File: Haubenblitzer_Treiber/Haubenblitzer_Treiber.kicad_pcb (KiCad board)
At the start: 2 copper layers, 75 x 60 mm, 40 parts, among them J1 ISCP, J2 Micro_USB, J3 Screw_Terminal_01x02, J4 Screw_Terminal_01x03, J5 Screw_Terminal_01x05, J6 RJ12, J7 RJ12, Q1 MMBT3906, Q2 MMBT3906, U1 ATmega32U4-AU, U2 NCV8460, U3 3021-D-E-1000, U4 3021-D-E-1000, U5 USBLC6-2P6, Y1 Crystal

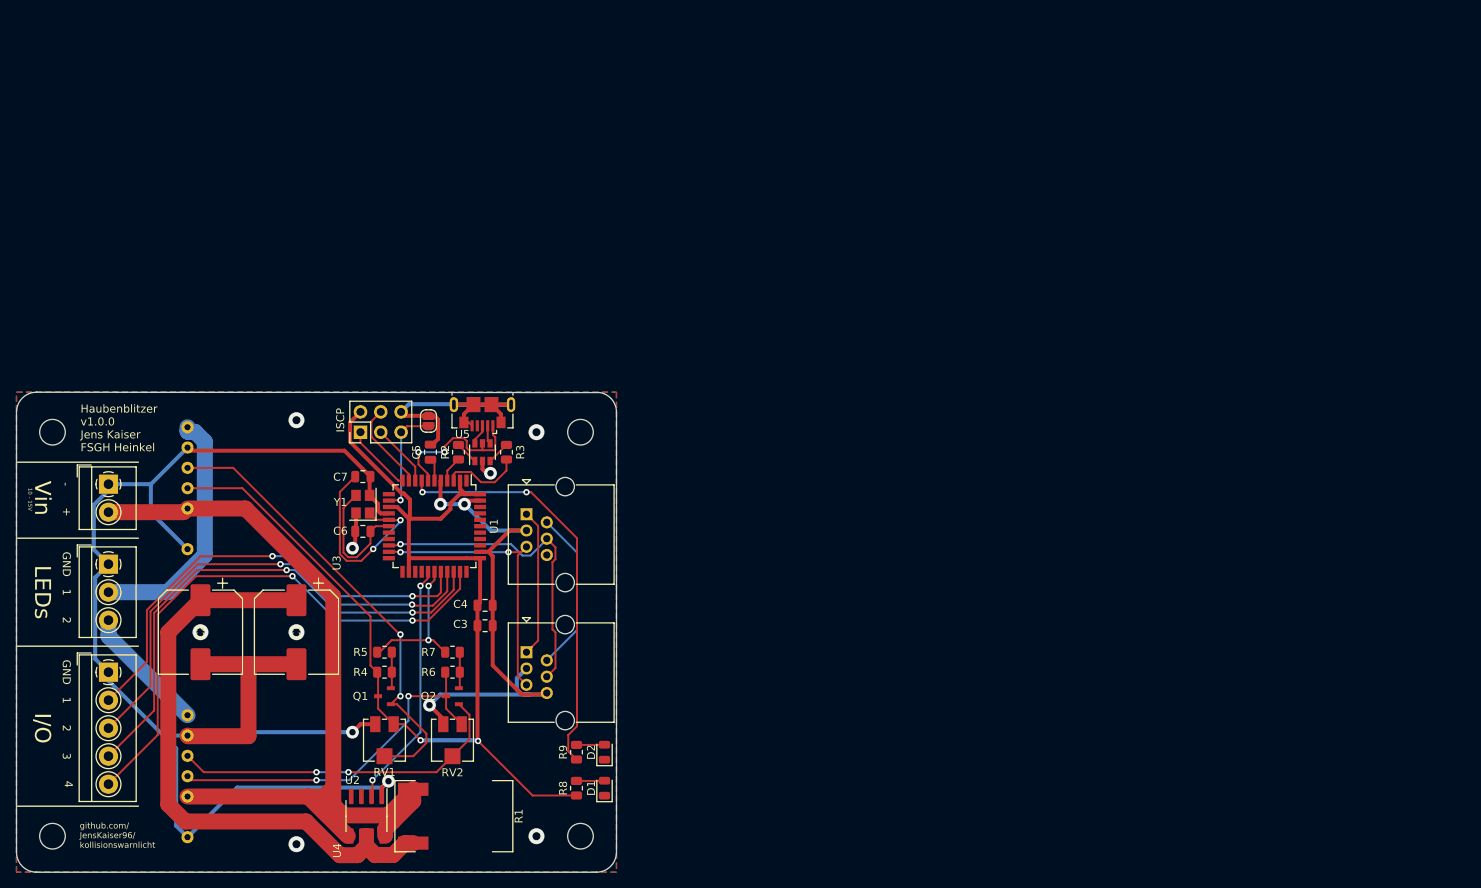
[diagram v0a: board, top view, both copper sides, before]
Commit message: Version2.0
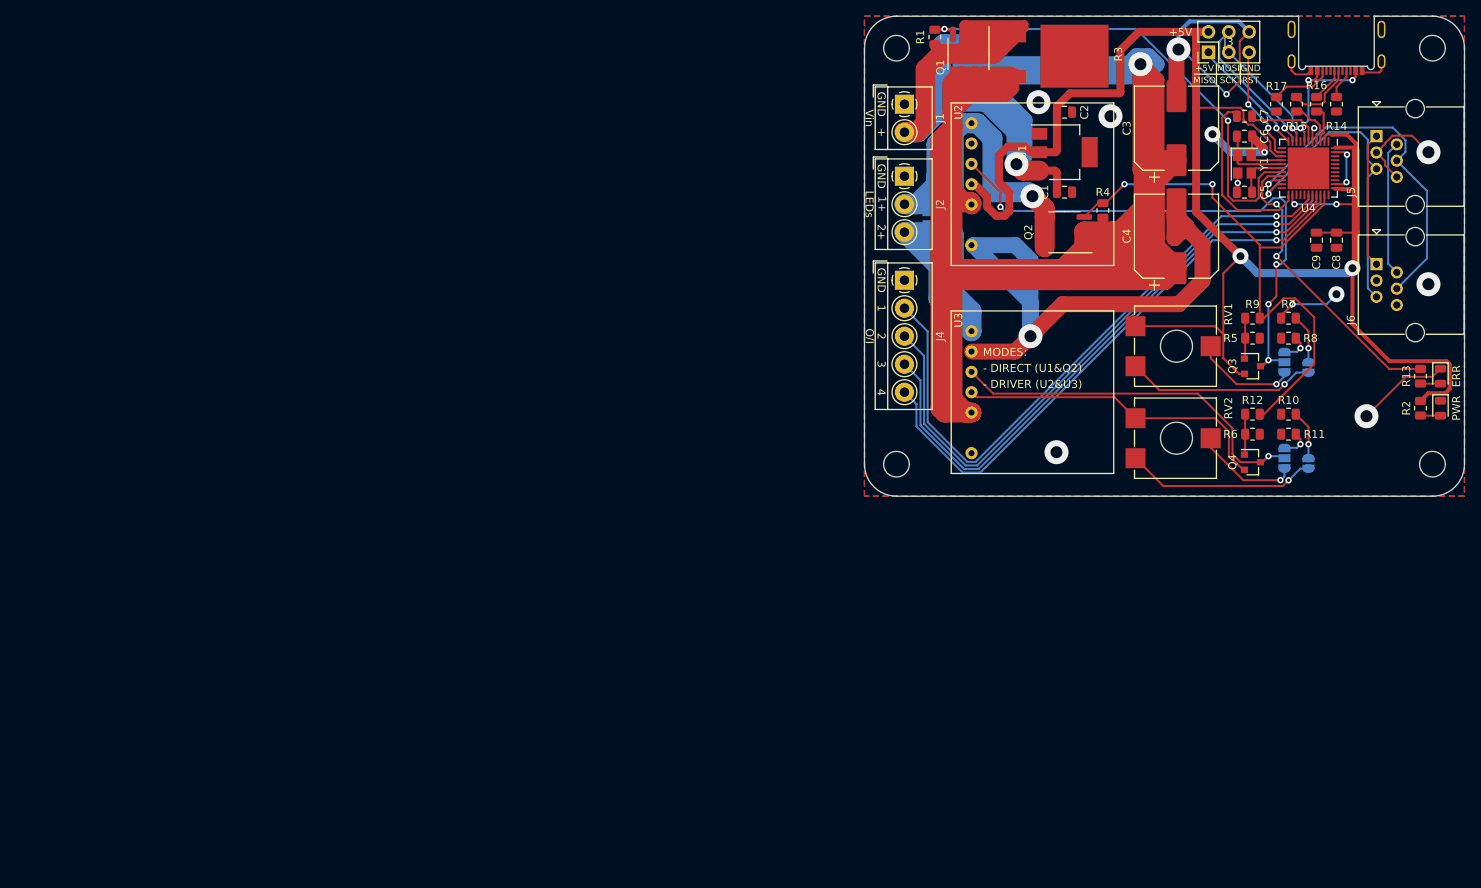
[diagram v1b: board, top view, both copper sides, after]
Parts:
- removed D1, D2: LED, LED_SMD:LED_0805_2012Metric
- removed U5: USBLC6-2P6, Package_TO_SOT_SMD:SOT-23-6
- added C8: 0.1uF, Capacitor_SMD:C_0805_2012Metric, F.Cu at (185.0, 111.0)
- added C9: 10uF, Capacitor_SMD:C_0805_2012Metric, F.Cu at (182.5, 111.0)
- added ERR: LED, LED_SMD:LED_0805_2012Metric, F.Cu at (198.0, 128.0)
- added JP2: Jumper, Jumper:SolderJumper-3_P1.3mm_Open_RoundedPad1.0x1.5mm, B.Cu at (178.5, 126.2)
- added JP3: Jumper, Jumper:SolderJumper-3_P1.3mm_Open_RoundedPad1.0x1.5mm, B.Cu at (178.5, 138.2)
- added JP4: Jumper, Jumper:SolderJumper-2_P1.3mm_Open_RoundedPad1.0x1.5mm, B.Cu at (181.5, 126.9)
- added JP5: Jumper, Jumper:SolderJumper-2_P1.3mm_Open_RoundedPad1.0x1.5mm, B.Cu at (181.5, 138.9)
- added JP6: Jumper, Jumper:SolderJumper-2_P1.3mm_Open_Pad2.0x4.0mm, B.Cu at (135.2, 108.2)
- added PWR: LED, LED_SMD:LED_0805_2012Metric, F.Cu at (198.0, 132.0)
- added Q3: AO3401A, Package_TO_SOT_SMD:SOT-23, F.Cu at (174.5, 126.8)
- added Q4: AO3401A, Package_TO_SOT_SMD:SOT-23, F.Cu at (174.5, 138.8)
- added R10: 1K, Resistor_SMD:R_0805_2012Metric, F.Cu at (179.0, 132.8)
- added R11: 5K, Resistor_SMD:R_0805_2012Metric, F.Cu at (179.0, 135.2)
- added R12: 5k, Resistor_SMD:R_0805_2012Metric, F.Cu at (174.5, 135.2)
- added R13: 220, Resistor_SMD:R_0805_2012Metric, F.Cu at (195.5, 128.0)
- added R14: 5.1K, Resistor_SMD:R_0805_2012Metric, F.Cu at (185.0, 94.0)
- added R15: 22, Resistor_SMD:R_0805_2012Metric, F.Cu at (180.0, 94.0)
- added R16: 22, Resistor_SMD:R_0805_2012Metric, F.Cu at (182.5, 94.0)
- added R17: 5.1K, Resistor_SMD:R_0805_2012Metric, F.Cu at (177.5, 94.0)
- C1: value 220uF -> 1uF; footprint Capacitor_SMD:CP_Elec_10x10 -> Capacitor_SMD:C_0805_2012Metric
- C2: value 220uF -> 4.7uF; footprint Capacitor_SMD:CP_Elec_10x10 -> Capacitor_SMD:C_0805_2012Metric
- C3: value 0.1uF -> 220uF; footprint Capacitor_SMD:C_0805_2012Metric -> Capacitor_SMD:CP_Elec_10x10
- C4: value 10uF -> 220uF; footprint Capacitor_SMD:C_0805_2012Metric -> Capacitor_SMD:CP_Elec_10x10
- C5: value 1uF -> 18pF
- C7: value 18pF -> 1uF
- J1: value ISCP -> Screw_Terminal; footprint Connector_PinHeader_2.54mm:PinHeader_2x03_P2.54mm_Vertical -> TerminalBlock_4Ucon:TerminalBlock_4Ucon_1x02_P3.50mm_Horizontal
- J2: value Micro_USB -> Screw_Terminal; footprint Connector_USB:USB_Micro-B_GCT_USB3076-30-A -> TerminalBlock_4Ucon:TerminalBlock_4Ucon_1x03_P3.50mm_Horizontal
- J3: value Screw_Terminal_01x02 -> ISCP; footprint TerminalBlock_4Ucon:TerminalBlock_4Ucon_1x02_P3.50mm_Horizontal -> Connector_PinHeader_2.54mm:PinHeader_2x03_P2.54mm_Vertical
- J4: value Screw_Terminal_01x03 -> Screw_Terminal; footprint TerminalBlock_4Ucon:TerminalBlock_4Ucon_1x03_P3.50mm_Horizontal -> TerminalBlock_4Ucon:TerminalBlock_4Ucon_1x05_P3.50mm_Horizontal
- J5: value Screw_Terminal_01x05 -> RJ12; footprint TerminalBlock_4Ucon:TerminalBlock_4Ucon_1x05_P3.50mm_Horizontal -> Connector_RJ:RJ25_Wayconn_MJEA-660X1_Horizontal
- J7: value RJ12 -> USB_C_4510; footprint Connector_RJ:RJ25_Wayconn_MJEA-660X1_Horizontal -> Connector_USB:USB_C_4510
- JP1: value Reset -> Jumper; footprint Jumper:SolderJumper-2_P1.3mm_Open_RoundedPad1.0x1.5mm -> Jumper:SolderJumper-2_P1.3mm_Open_Pad2.0x4.0mm; moved to B.Cu
- Q1, Q2: value MMBT3906 -> IRF7205; footprint Package_TO_SOT_SMD:SA1162 -> Package_SO:SOIC-8_IRF7205
- R1: value 5 -> 10k; footprint Resistor_SMD:MP725 -> Resistor_SMD:R_0805_2012Metric
- R2: value 22 -> 220
- R3: value 22 -> 5; footprint Resistor_SMD:R_0805_2012Metric -> Package_TO_SOT_SMD:PAK-2
- R4: value 5k -> 10k
- R5, R6: value 5k -> 200
- R7: value 5k -> 5K
- R8, R9: value 220 -> 5k
- RV1, RV2: footprint Potentiometer_SMD:Potentiometer_Vishay_TS53YJ_Vertical -> Potentiometer_SMD:Potentiometer_ACP_PS10_Vertical_Hole
- U1: value ATmega32U4-AU -> LDL1117S50R; footprint Package_QFP:TQFP-44_10x10mm_P0.8mm -> Package_TO_SOT_SMD:SOT-223
- U2: value NCV8460 -> 3021-D-E-1000; footprint Package_SO:SOIC-8_3.9x4.9mm_P1.27mm -> Converter_DCDC:3021-D-E-1000
- U4: value 3021-D-E-1000 -> ATmega16U4-AU; footprint Converter_DCDC:3021-D-E-1000 -> Package_DFN_QFN:QFN-44-1EP_7x7mm_P0.5mm_EP5.2x5.2mm
- moved J5 172.1 mm to (190.0, 98.0), turned to 90 degrees
- moved U4 152.7 mm to (181.5, 102.0), turned to 270 degrees
- moved J3 147.7 mm to (169.0, 87.5), turned to 90 degrees
- moved C2 126.1 mm to (151.0, 95.0), turned to 180 degrees
- moved J7 125.0 mm to (185.0, 89.2), turned to 180 degrees
- moved C6 120.8 mm to (173.5, 98.0), turned to 180 degrees
- moved R2 120.4 mm to (195.5, 132.0), turned to 270 degrees
- moved C7 119.1 mm to (173.5, 95.5)
- moved Y1 118.1 mm to (173.5, 101.5), turned to 270 degrees
- moved H2 116.8 mm to (197.0, 87.0)
- moved R5 116.3 mm to (174.5, 120.8)
- moved H4 116.2 mm to (197.0, 139.0)
- moved R1 116.2 mm to (134.8, 85.6), turned to 90 degrees
- moved H1 115.9 mm to (130.0, 87.0)
- moved H3 115.3 mm to (130.0, 139.0)
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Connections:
- C1 pad 1: Net-(C1-Pad1) -> GND
- C1 pad 2: GND -> VCC
- C2 pad 1: Net-(C1-Pad1) -> GND
- C2 pad 2: GND -> +5V
- C3 pad 1: GND -> /U_Driver
- C3 pad 2: LED1_Ref -> GND
- C4 pad 1: GND -> /U_Driver
- C4 pad 2: LED1_Ref -> GND
- C5 pad 2: U_cap -> /CLK_1
- C6 pad 2: CLK_1 -> /CLK_2
- C7 pad 1: CLK_2 -> GND
- C7 pad 2: GND -> Net-(C7-Pad2)
- J1 pad 1: MISO -> GND
- J1 pad 2: LED1_Ref -> VCC
- J2 pad 1: U_bus -> /GND_LED
- J2 pad 2: Net-(J2-Pad2) -> /U_LED1
- J2 pad 3: Net-(J2-Pad3) -> /U_LED2
- J3 pad 1: GND -> /MISO
- J3 pad 2: +12V -> +5V
- J4 pad 2: LED1_U+ -> /IO_MISC1
- J4 pad 3: LED2_U+ -> /IO_MISC2
- J5 pad 1: GND -> /RJ12_V1
- J5 pad 2: IO_misc1 -> /RJ12_V2
- J5 pad 3: IO_misc2 -> GND
- J5 pad 4: IO_misc3 -> /RX
- J5 pad 5: IO_misc4 -> /TX
- J6 pad 1: RJ12_V1 -> /RJ12_V1
- J6 pad 2: RJ12_V2 -> /RJ12_V2
- J6 pad 4: RX -> /RX
- J6 pad 5: TX -> /TX
- JP1 pad 1: GND -> VCC
- JP1 pad 2: RESET -> /U_Driver
- Q1 pad 1: LED1_Ctrl -> /U_Driver
- Q1 pad 2: Net-(Q1-Pad2) -> /IO_BRIDGE_INRUSH_R
- Q1 pad 3: LED1_Ref -> VCC
- Q2 pad 1: LED2_Ctrl -> /U_LED1
- Q2 pad 2: Net-(Q2-Pad2) -> /IO_LED
- Q2 pad 3: LED2_Ref -> /U_Driver
- R1 pad 1: +12V -> VCC
- R1 pad 2: Net-(C1-Pad1) -> /IO_BRIDGE_INRUSH_R
- R2 pad 1: D+ -> +5V
- R3 pad 1: Net-(R3-Pad1) -> VCC
- R3 pad 2: D- -> /U_Driver
- R4 pad 1: LED1_Ref -> /U_Driver
- R4 pad 2: Net-(Q1-Pad2) -> /IO_LED
- R5 pad 1: Net-(Q1-Pad2) -> /IO_LED
- R5 pad 2: IO_LED -> Net-(Q3-Pad1)
- R6 pad 1: LED2_Ref -> /IO_LED
- R6 pad 2: Net-(Q2-Pad2) -> Net-(Q4-Pad1)
- R7 pad 1: Net-(Q2-Pad2) -> Net-(JP4-Pad2)
- R7 pad 2: IO_LED -> GND
- R8 pad 1: LED1_Ref -> Net-(JP2-Pad3)
- R8 pad 2: Net-(D1-Pad2) (its old number) -> GND
- R9 pad 1: RX_LED -> Net-(Q3-Pad1)
- R9 pad 2: Net-(D2-Pad2) -> GND
- RV1 pad 1: GND -> Net-(JP4-Pad1)
- RV1 pad 2: LED1_Ctrl -> Net-(JP2-Pad1)
- RV1 pad 3: LED1_Ref -> +5V
- RV2 pad 1: GND -> Net-(JP5-Pad1)
- RV2 pad 2: LED2_Ctrl -> Net-(JP3-Pad1)
- RV2 pad 3: LED2_Ref -> /LED2_REF
- U1 pad 1: Net-(U1-Pad1) -> GND
- U1 pad 2: LED1_Ref -> +5V
- U1 pad 3: D- -> VCC
- U1 pad 4: D+ -> (no net)
- U2 pad 1: GND -> /U_LED1
- U2 pad 2: IO_FETctrl -> GND
- U2 pad 3: Net-(U2-Pad3) -> /LED1_CTRL
- U2 pad 4: Net-(U2-Pad4) -> +5V
- U2 pad 5: +12V -> /U_Driver
- U2 pad 6: Net-(C1-Pad1) -> GND
- U3 pad 1: LED1_U+ -> /U_LED2
- U3 pad 3: LED1_Ctrl -> /LED2_CTRL
- U3 pad 4: LED1_Ref -> /LED2_REF
- U3 pad 5: +12V -> /U_Driver
- U4 pad 1: LED2_U+ -> Net-(U4-Pad1)
- U4 pad 2: GND -> +5V
- U4 pad 3: LED2_Ctrl -> /D-
- U4 pad 4: LED2_Ref -> /D+
- U4 pad 5: +12V -> GND
- U4 pad 6: GND -> Net-(C7-Pad2)
- Y1 pad 1: CLK_2 -> /CLK_2
- Y1 pad 3: CLK_1 -> /CLK_1
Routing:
- net /U_Driver: track 0.00 -> 333.6 mm, vias 0 -> 1
- net +5V: track 0.00 -> 213.2 mm, vias 0 -> 4
- net LED1_Ref: track 142.2 -> 0.00 mm, vias 2 -> 0
- net VCC: track 0.00 -> 112.3 mm, vias 0 -> 1
- net +12V: track 110.2 -> 0.00 mm
- net Net-(C1-Pad1): track 93.4 -> 0.00 mm
- net GND: track 303.1 -> 210.7 mm, vias 13 -> 17
- net /IO_MISC1: track 0.00 -> 79.3 mm, vias 0 -> 1
- net /IO_MISC2: track 0.00 -> 77.1 mm, vias 0 -> 1
- net /IO_MISC3: track 0.00 -> 74.9 mm, vias 0 -> 1
- net /IO_MISC4: track 0.00 -> 72.7 mm, vias 0 -> 1
- net /IO_LED: track 0.00 -> 72.4 mm, vias 0 -> 2
- net IO_misc4: track 69.6 -> 0.00 mm, vias 2 -> 0
- net /LED1_CTRL: track 0.00 -> 68.0 mm, vias 0 -> 4
- net IO_misc3: track 65.6 -> 0.00 mm, vias 2 -> 0
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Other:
- outline, holes or cut-outs redrawn
- board text added: "+5V"
- board text added: "- DIRECT (U1&Q2)"
- board text added: "- DRIVER (U2&U3)"
- board text added: "1+"
- board text added: "2+"
- board text added: "CTRL"
- board text added: "DRIVER MODE: I adj/max"
- board text added: "LED+"
- board text added: "LED-"
- board text added: "MISO"
- board text added: "MODES:"
- board text added: "MOSI"
- board text added: "Overcurrent Protection: ◼:OFF ◻:ON"
- board text added: "REF"
- board text added: "RST"
- board text added: "SCK"
- board text added: "Vin+"
- board text added: "Vin-"
- board text added: "adj. I LED1"
- board text added: "adj. I LED2"
- board text added: "adj:"
- board text added: "max:"
- board text added: "◼: only when set to max"
- board text removed: "-"
- board text removed: "10 - 15V"
- board text removed: "Haubenblitzer v1.0.0 Jens Kaiser FSGH Heinkel"
- board text removed: "ISCP"
- board text removed: "github.com/ JensKaiser96/ kollisionswarnlicht"
